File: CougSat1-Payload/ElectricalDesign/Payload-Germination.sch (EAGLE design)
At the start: 9 parts, among them J1 CougSat Card, J2 Germination Chamber, Q1 CSD25402Q3A, Q2 CSD25402Q3A, U1 TXS0102DQM, U2 TXS0102DQM, U3 TXS0102DQM

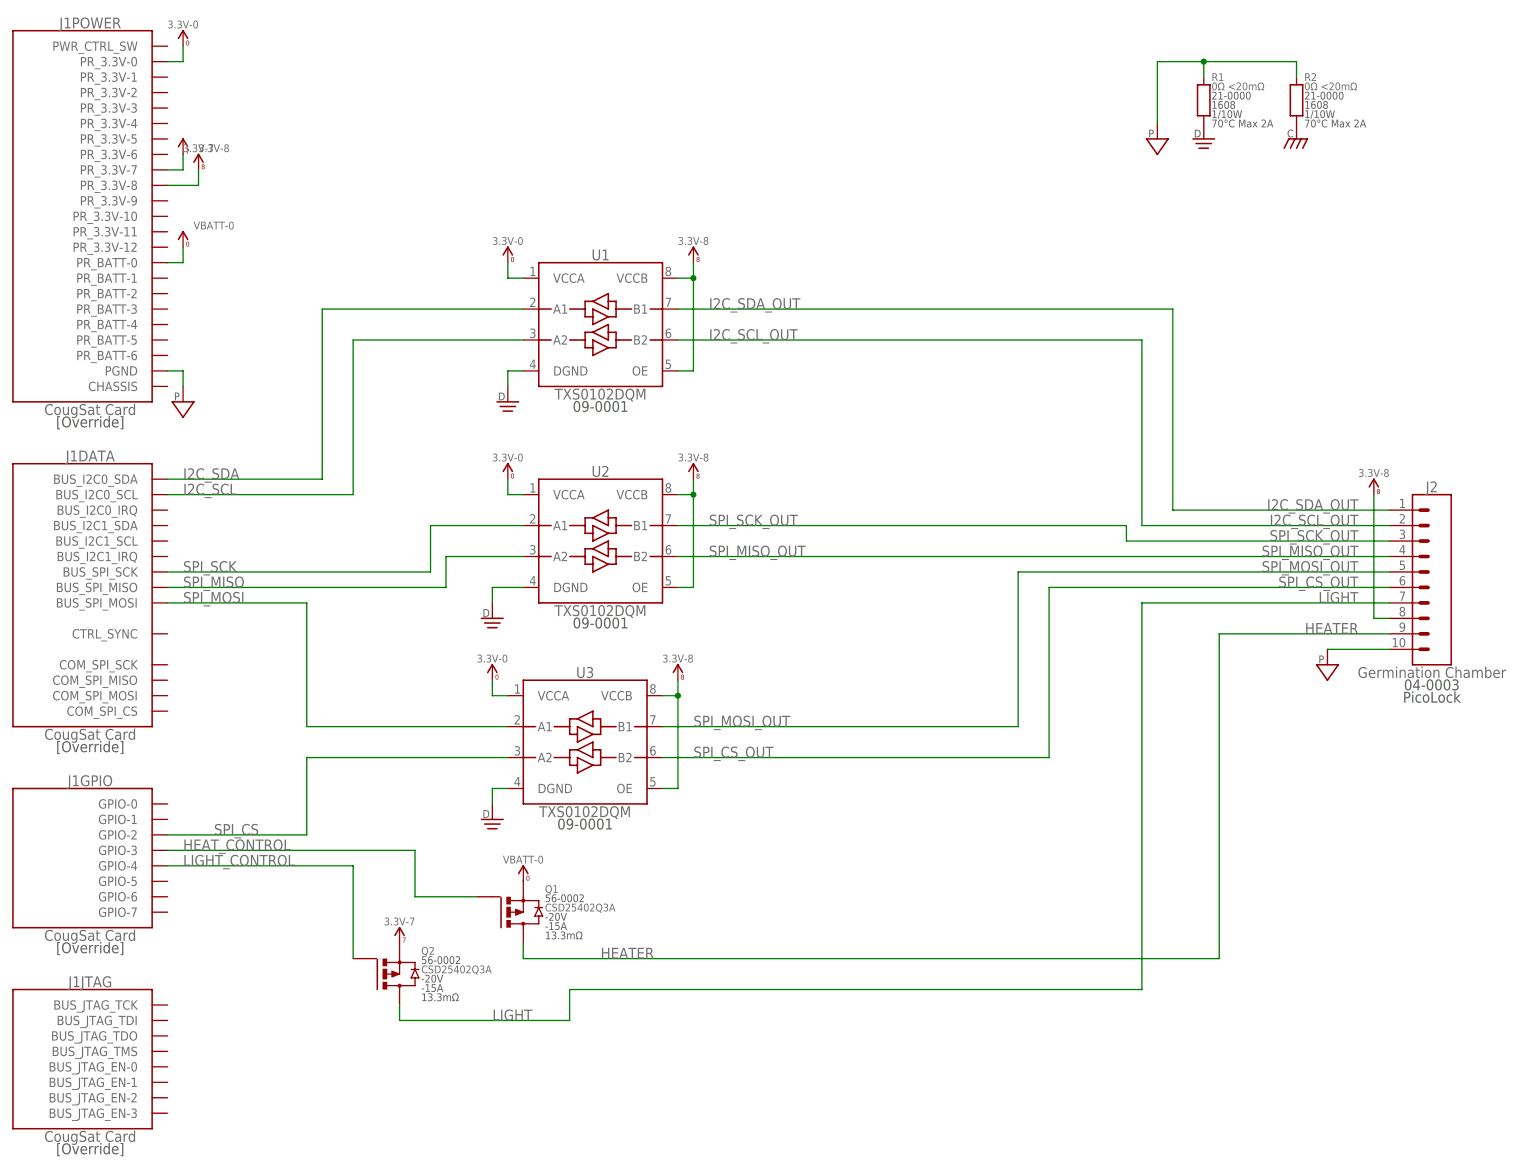
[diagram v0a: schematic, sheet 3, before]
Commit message: Fixed Formatting
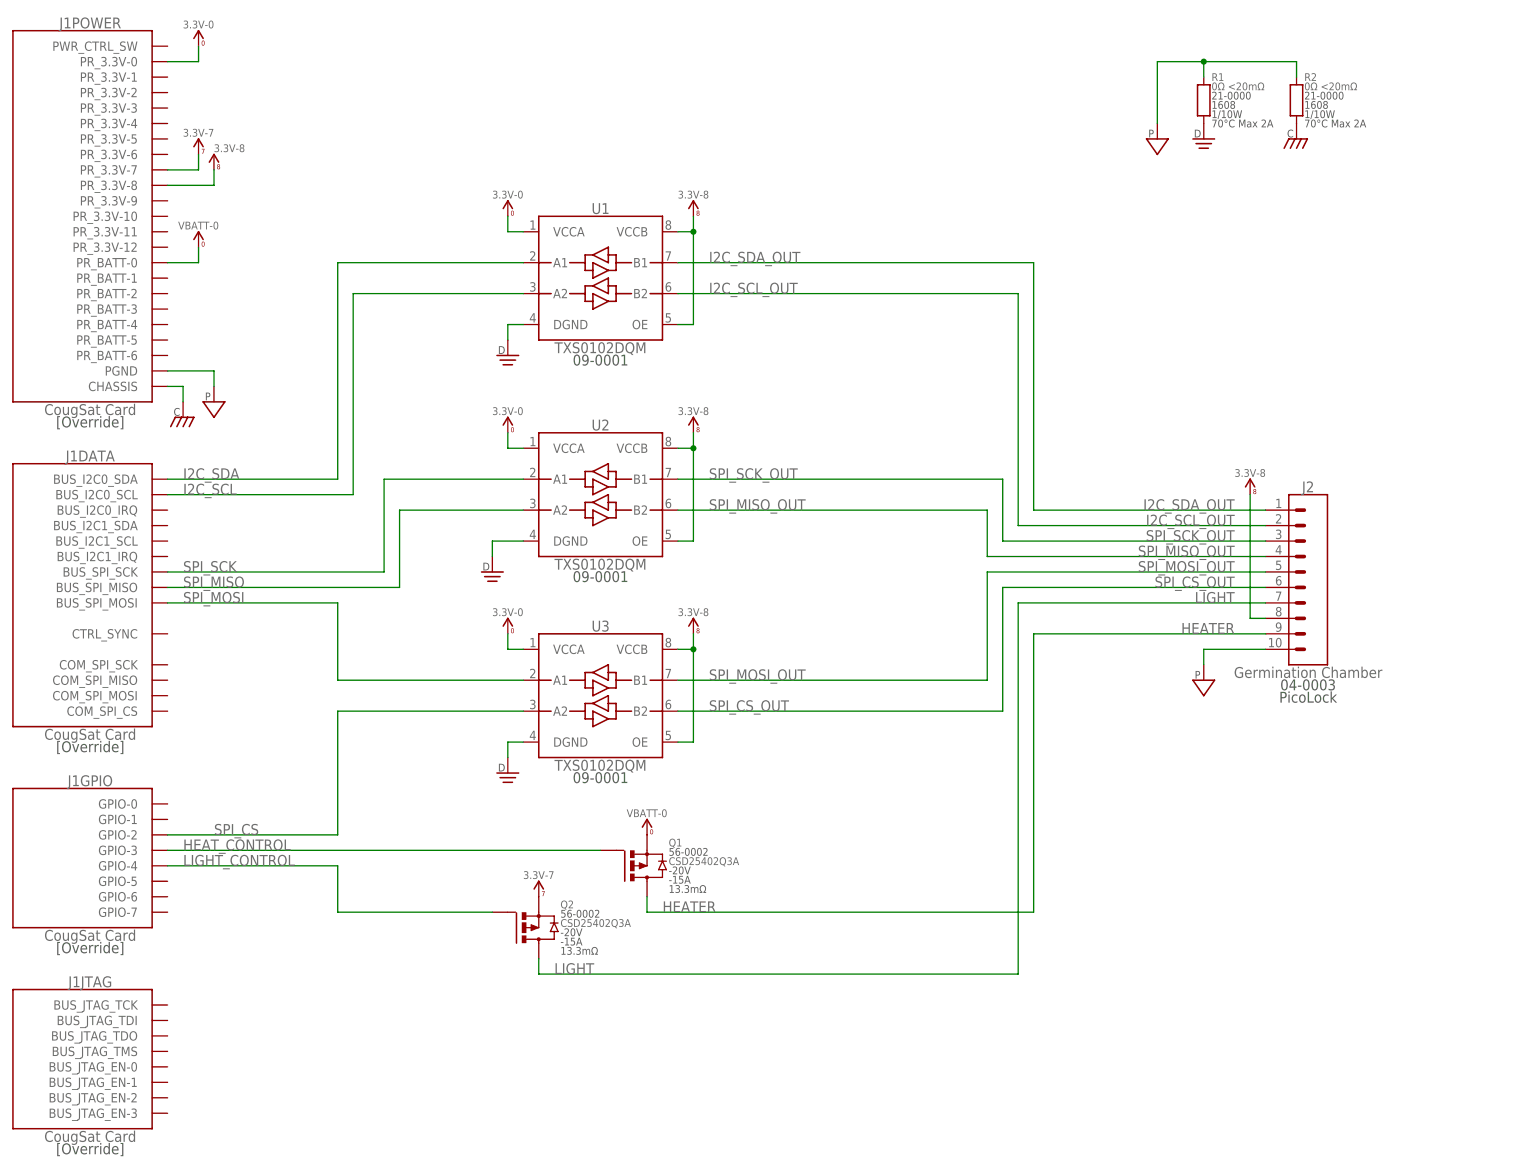
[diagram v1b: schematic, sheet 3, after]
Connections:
- net CHASSIS: now also J1POWER.CHASSIS
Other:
- moved on the sheet: J2, Q1, Q2, U1, U2, U3
